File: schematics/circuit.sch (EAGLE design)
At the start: 17 parts, among them U1 AD5241BRU1M-REEL7AD5241BRZ1M, U3 ADXL375BCCZ, X1 87758-1816

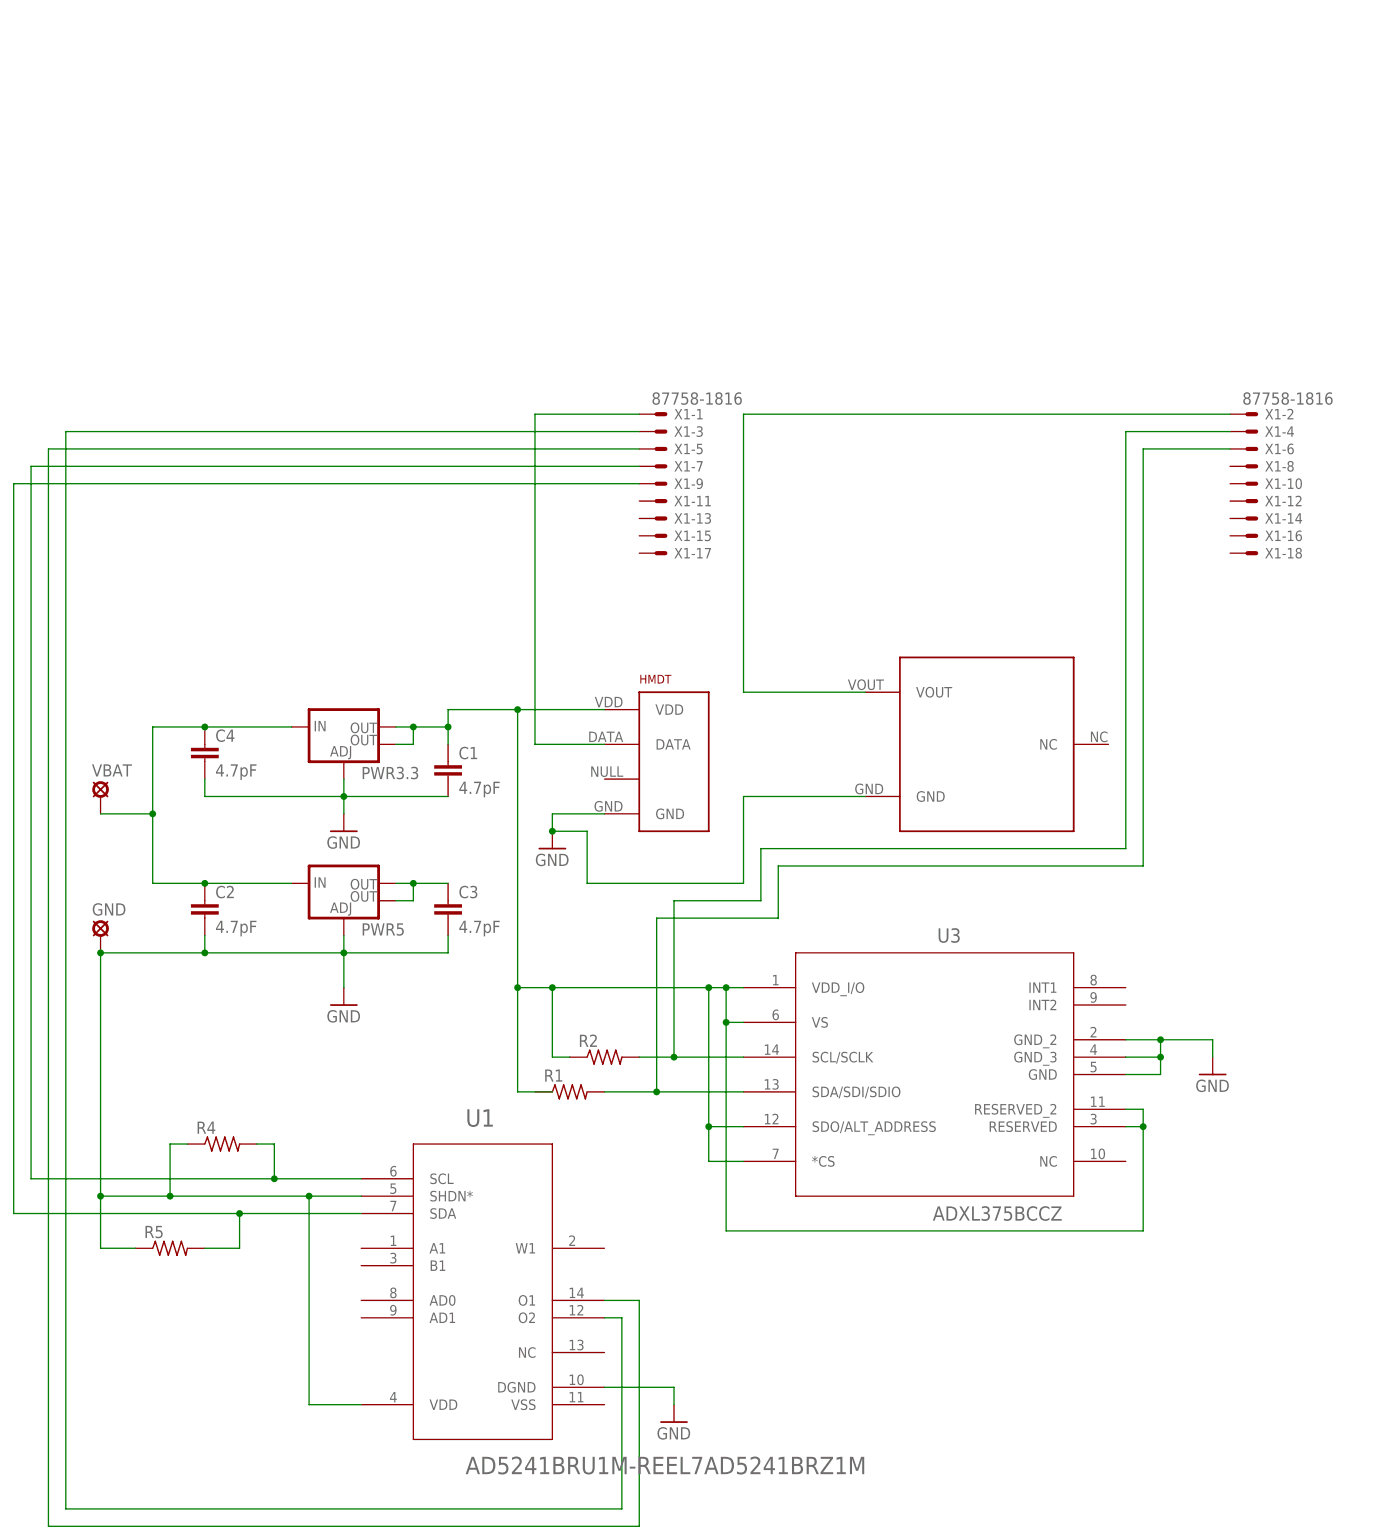
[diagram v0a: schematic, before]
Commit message: исправлена схема
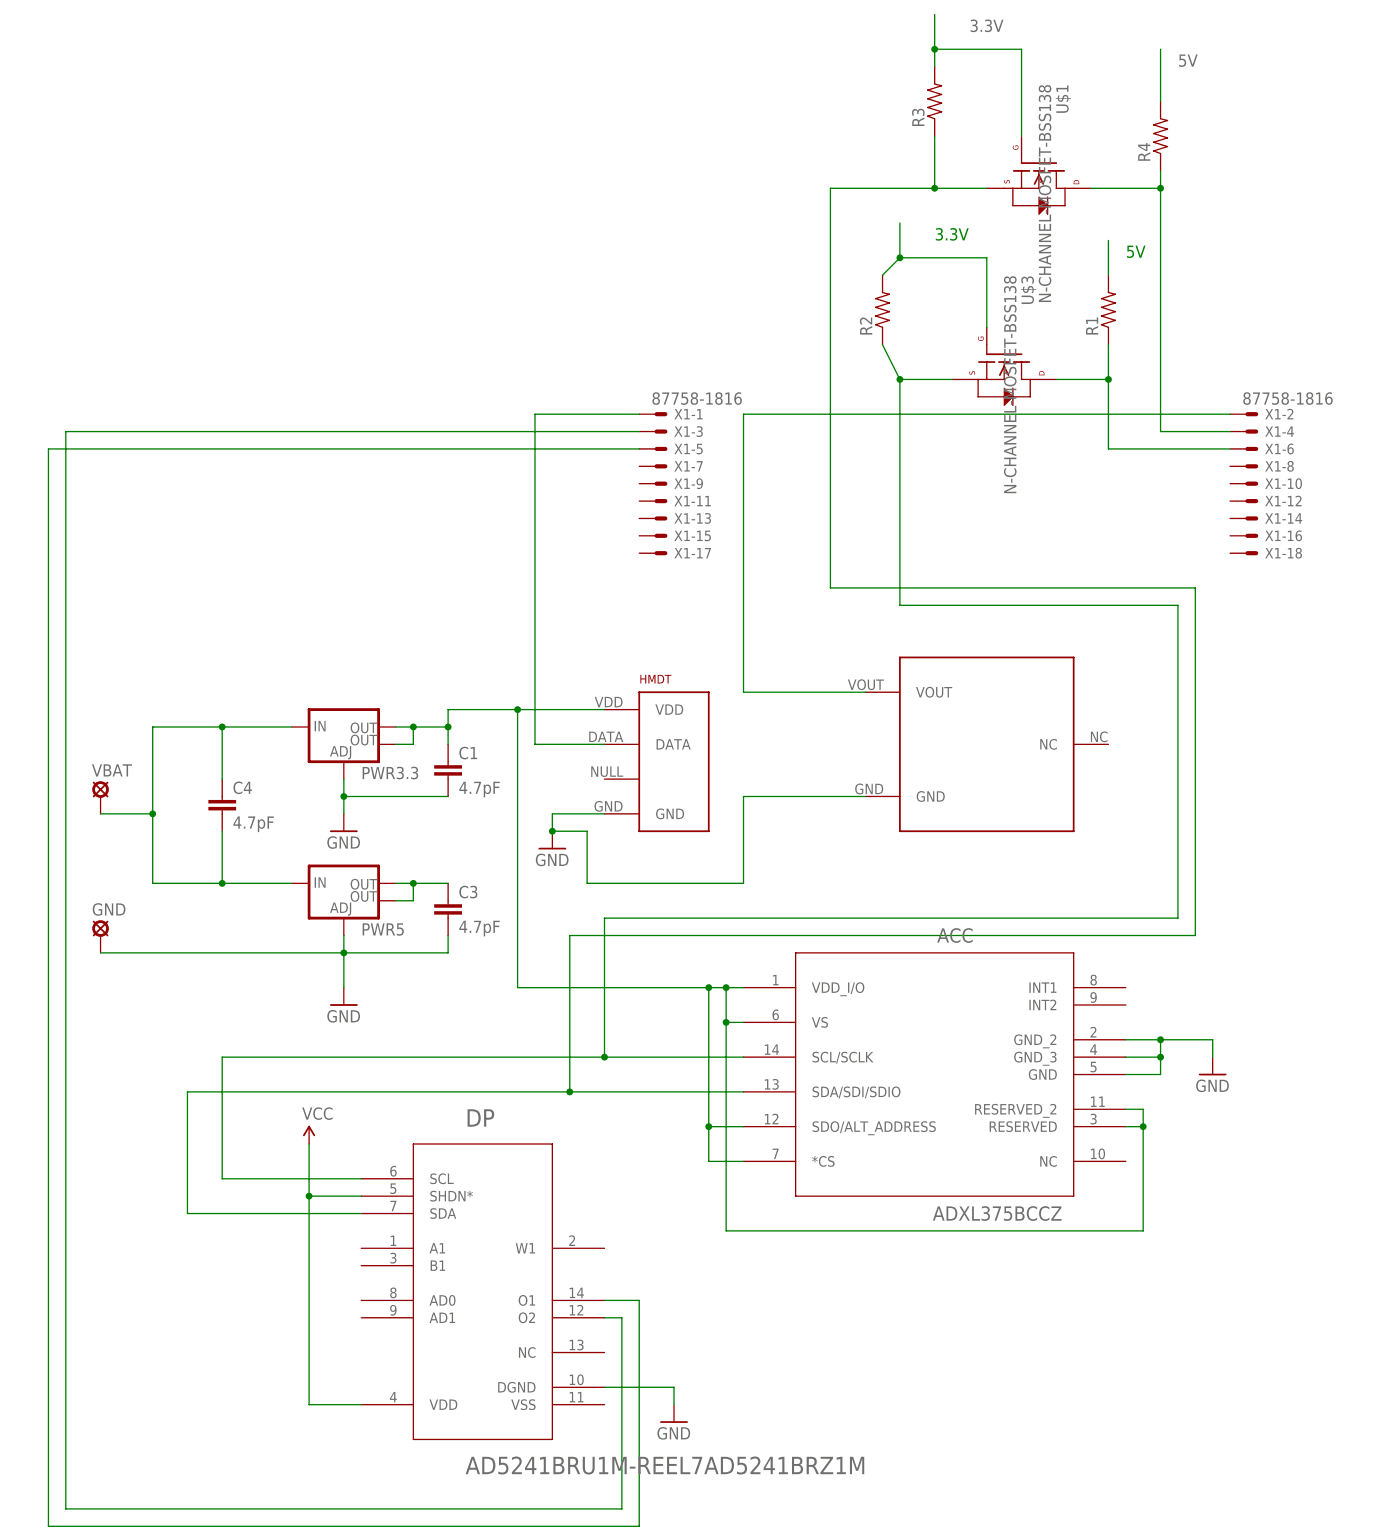
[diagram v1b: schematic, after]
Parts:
- removed C2: 4.7pF, SparkFun-Capacitors:4.7PF-50V(-/+.25PF)(0603)
- removed R5: (no value), rcl:R-US_0207/10
- added R3: (no value), SparkFun-Passives:RESISTOR0402-RES
- added U$1, U$3: N-CHANNEL-MOSFET-BSS138, GeekAmmo:N-CHANNEL-MOSFET-BSS138
- R1, R2, R4: device rcl:R-US_0207/10 -> SparkFun-Passives:RESISTOR0402-RES
- renumbered U1 to DP, U3 to ACC
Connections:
- removed net N$3: DP.SCL, R4.2, X1-7.S
- removed net N$5: DP.SDA, R5.2, X1-9.S
- removed net N$7: ACC.SCL/SCLK, R2.2, X1-4.S
- removed net N$8: ACC.SDA/SDI/SDIO, R1.2, X1-6.S
- new net SCL3.3V: ACC.SCL/SCLK, DP.SCL, R2.1, U$3.S
- new net SCL5V: R1.1, U$3.D, X1-6.S
- new net SDA3.3V: ACC.SDA/SDI/SDIO, DP.SDA, R3.1, U$1.S
- new net SDA5V: R4.1, U$1.D, X1-4.S
- new net VCC: DP.SHDN*, DP.VDD
- net 3.3V: now also R2.2, R3.2, U$1.G, U$3.G; no longer R2.1
- net 5V: now also R1.2, R4.2
- net GND: no longer C2.2, C4.2, DP.SHDN*, DP.VDD, R4.1, R5.1
- net VBAT: now also C4.2; no longer C2.1
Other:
- note added: "3.3V"
- note added: "5V"
- note added: "SCL"
- note added: "SDA"
- moved on the sheet: C4, R1, R2, R4
